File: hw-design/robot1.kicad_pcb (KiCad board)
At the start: 2 copper layers, 63.5 x 26.7 mm, 75 parts, among them P1 test-double, P2 CONN_01X04, P3 CONN_01X03, P4 left_motor, P5 right_motor, P6 CONN_01X05, P7 CONN_01X05, U1 STM32F072CB / STM32F042C6, U2 usb-micro, U3 MCP73833, U4 AP111733, U5 drv8835, U6 drv8835, U7 BlueNRG, U8 BALF-NRG-01D3, Y1 16MHz, Y2 32kHz, Y3 16MHz

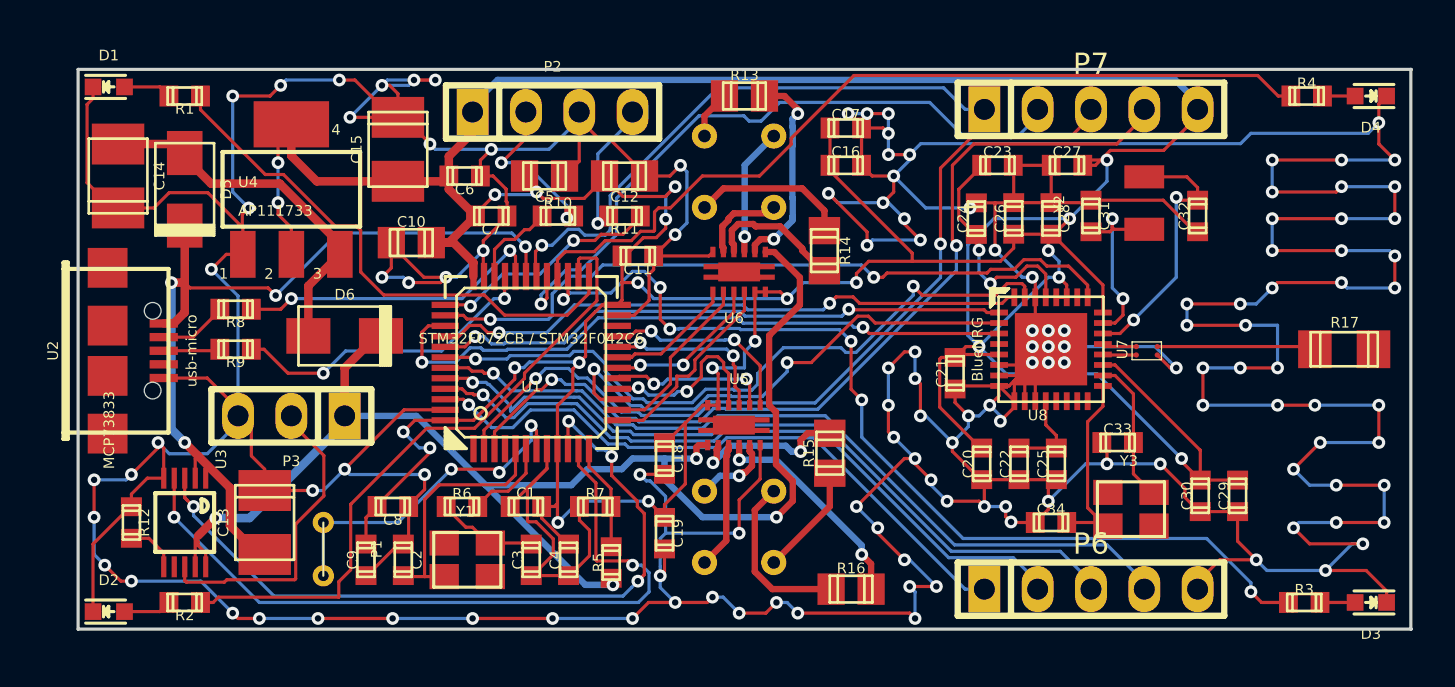
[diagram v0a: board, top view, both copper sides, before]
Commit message: Mounting holes for additional wheels or whatever
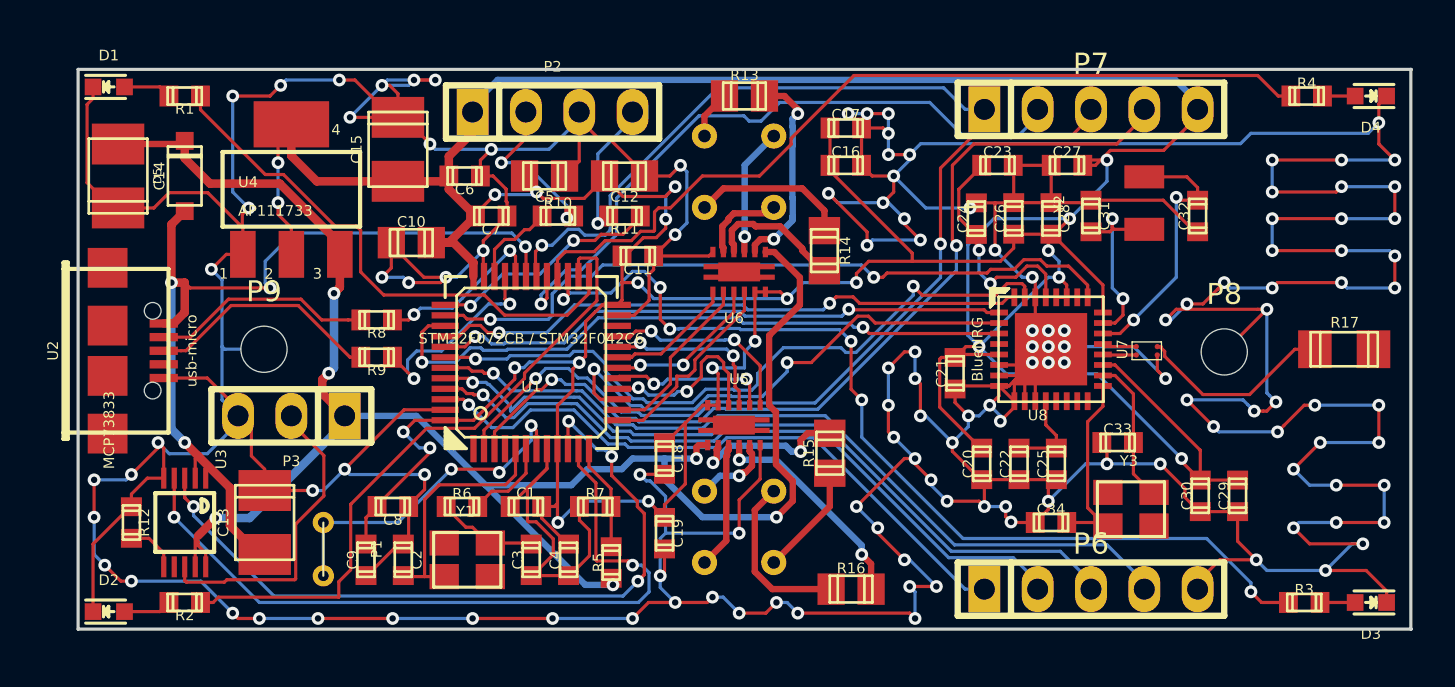
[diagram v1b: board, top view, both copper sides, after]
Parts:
- removed D6: D_Schottky, w_smd_diode:do214ac
- added P8: CONN_01X01, Mounting_Holes:MountingHole_2.2mm_M2_ISO7380, F.Cu at (195.6, 129.0)
- added P9: CONN_01X01, Mounting_Holes:MountingHole_2.2mm_M2_ISO7380, F.Cu at (149.8, 128.9)
- D5: footprint w_smd_diode:do214ac -> iwasz:sod123-pins21
- moved R8 6.74 mm to (155.2, 127.5)
- moved R9 6.73 mm to (155.2, 129.3)
- moved D5 0.63 mm to (146.1, 120.7), turned to 90 degrees
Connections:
- C14 pad 1: Net-(C14-Pad1) -> +BATT
- D5 pad 1: Net-(C14-Pad1) -> +BATT
- U4 pad 3: Net-(C14-Pad1) -> +BATT
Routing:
- net Net-(C14-Pad1): track 17.7 -> 0.00 mm
- net +BATT: track 67.5 -> 85.0 mm, vias 4 -> 6
- net GND: track 496.2 -> 506.5 mm
- net Net-(R9-Pad1): track 2.70 -> 11.3 mm
- net Net-(R8-Pad1): track 3.25 -> 10.6 mm
- net Net-(R8-Pad2): track 14.8 -> 8.31 mm
- net Net-(R9-Pad2): track 15.1 -> 9.87 mm
- net Net-(R17-Pad2): track 7.62 -> 9.52 mm
- net +5V: track 42.7 -> 44.4 mm
